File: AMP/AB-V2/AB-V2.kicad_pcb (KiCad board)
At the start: 2 copper layers, 129.9 x 70.2 mm, 52 parts, among them J1 AUX, J3 AUX, P1 WJ500V-5.08-3P, Q1 2SC5200N-OSEN, Q13 BD140, Q14 BD140, Q15 BD139, Q16 BD139, Q17 BD140, Q18 BD140, Q2 2SC5200N-OSEN, Q21 BD139, U1 CYA0630-4.7UH

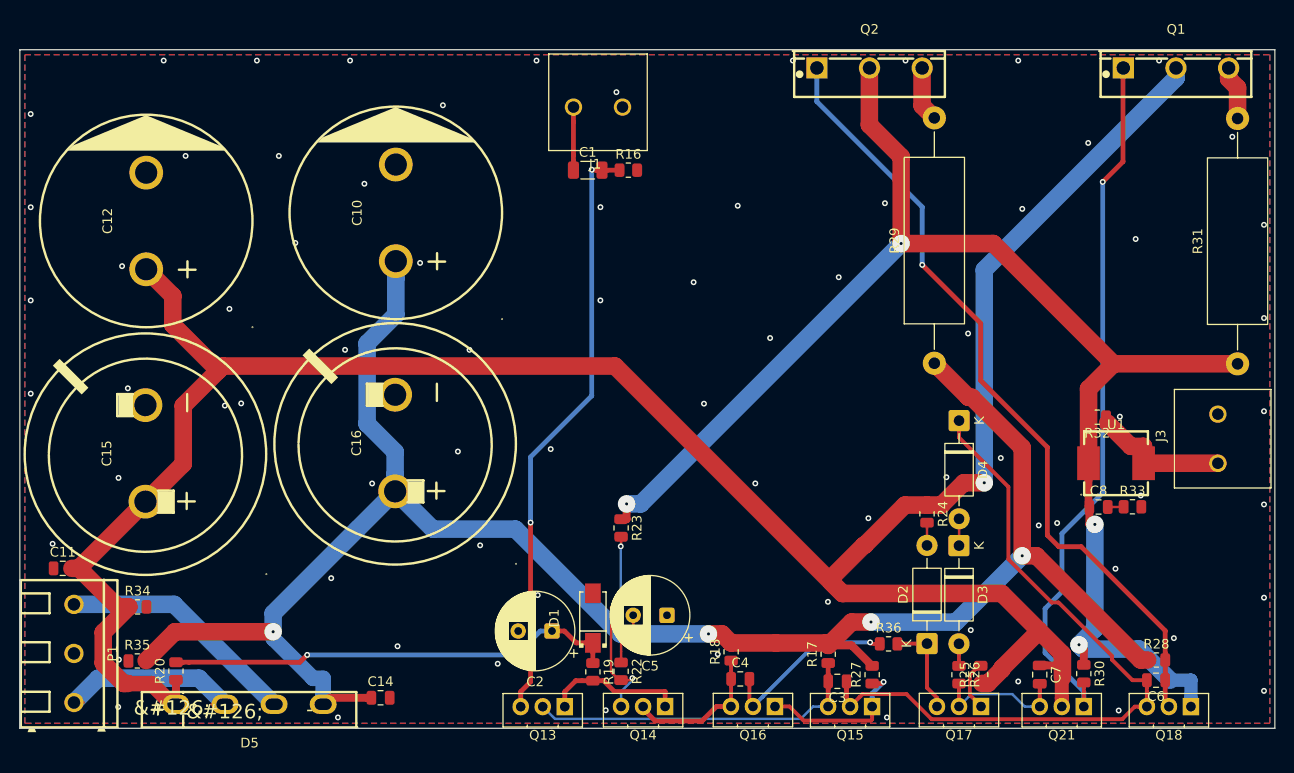
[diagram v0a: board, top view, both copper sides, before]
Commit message: kfahh
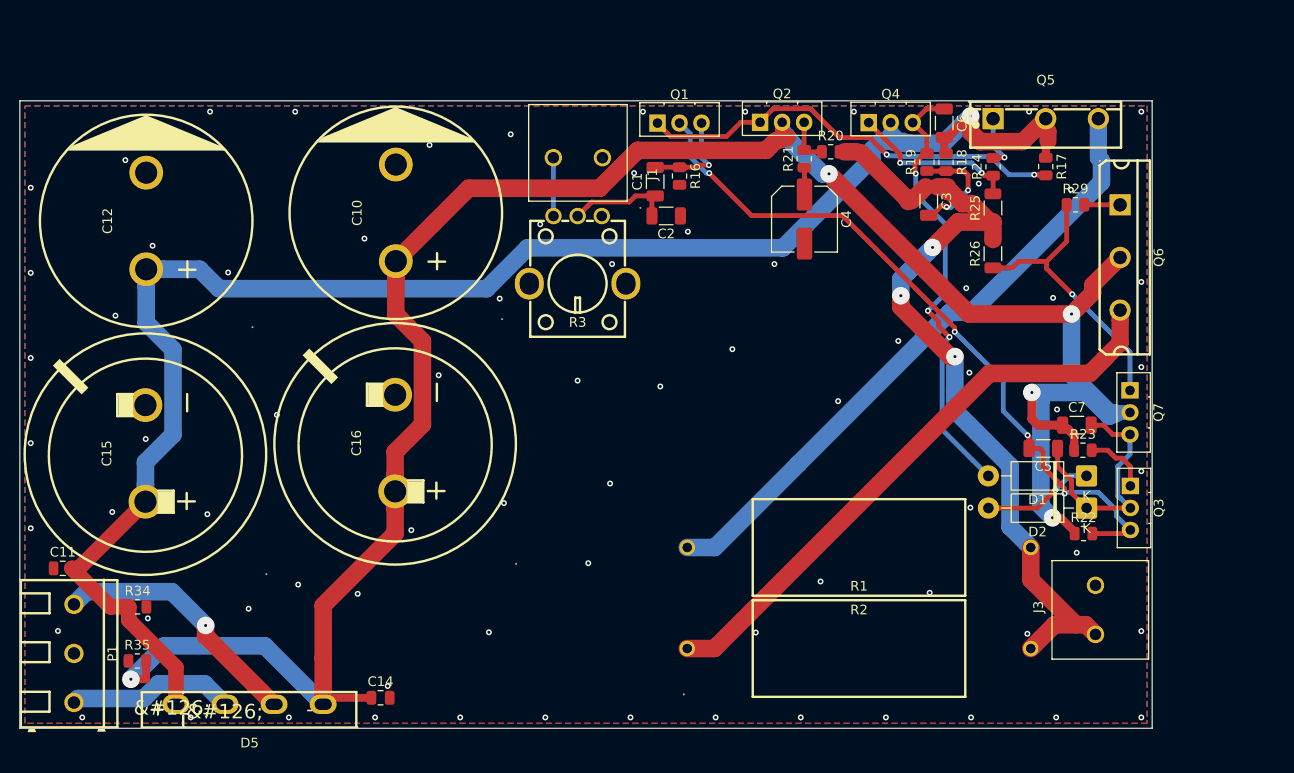
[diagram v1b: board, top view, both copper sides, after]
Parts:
- removed C8: 100 nF, Capacitor_SMD:C_0805_2012Metric
- removed D3, D4: 1N4007, Diode_THT:D_DO-41_SOD81_P10.16mm_Horizontal
- removed Q13, Q14, Q17, Q18: BD140, Package_TO_SOT_THT:TO-126-3_Vertical
- removed Q15, Q16, Q21: BD139, Package_TO_SOT_THT:TO-126-3_Vertical
- removed R27: 150, Resistor_SMD:R_0805_2012Metric
- removed R28, R30: 100, Resistor_SMD:R_0805_2012Metric
- removed R31: 0.47, Resistor_THT:R_Axial_DIN0617_L17.0mm_D6.0mm_P25.40mm_Horizontal
- removed R32, R33: 10, Resistor_SMD:R_0805_2012Metric
- removed R36: 10k, Resistor_SMD:R_0805_2012Metric
- removed U1: CYA0630-4.7UH, lcsc_footprints:C5189748_IND-SMD_L7_2-W6_6_GPSR07X0
- added Q3: BD139, Package_TO_SOT_THT:TO-126-3_Vertical, F.Cu at (245.0, 85.0)
- added Q4: BD139, Package_TO_SOT_THT:TO-126-3_Vertical, F.Cu at (217.9, 47.4)
- added Q5: 2SC5200N-OSEN, lcsc_footprints:C49055716_TO-3P-3_L15_6-W4_8-P5_45-L, F.Cu at (236.2, 47.0)
- added Q6: 2SA1943-O(Q, lcsc_footprints:C545244_TO-3PL_L20_0-W5_0-P5_45-L_1, F.Cu at (243.9, 61.4)
- added Q7: BD140, Package_TO_SOT_THT:TO-126-3_Vertical, F.Cu at (244.9, 75.2)
- added R1: CR-L5W-0.33ΩJ, lcsc_footprints:C334290_RES-TH_BD9_5-L22_0-P26_00-D0_7, F.Cu at (216.9, 91.4)
- added R2: CR-L5W-0.33ΩJ, lcsc_footprints:C334290_RES-TH_BD9_5-L22_0-P26_00-D0_7, F.Cu at (216.9, 101.9)
- added R21: 470, Resistor_SMD:R_0805_2012Metric, F.Cu at (211.2, 51.2)
- added R3: RK09K1130A70, lcsc_footprints:C351173_RES-TH_RK09K1130A70, F.Cu at (187.8, 60.6)
- C1: value 2.2 uF -> 10 uF
- C2, C5: value 100 uF -> 100 pF; footprint Capacitor_THT:CP_Radial_D8.0mm_P3.50mm -> Capacitor_SMD:C_1206_3216Metric
- C3: value 10 pF -> 10 uF; footprint Capacitor_SMD:C_0805_2012Metric -> Capacitor_SMD:C_1206_3216Metric
- C4: value 10 pF -> 100 uF; footprint Capacitor_SMD:C_0805_2012Metric -> Capacitor_SMD:C_Elec_6.3x7.7
- C6, C7: value 1 nF -> 470 pF; footprint Capacitor_SMD:C_0805_2012Metric -> Capacitor_SMD:C_1206_3216Metric
- D1: value 1SMA4749A -> 1N4007; footprint lcsc_footprints:C173489_SMA_L4_4-W2_8-LS5_4-RD -> Diode_THT:D_DO-41_SOD81_P10.16mm_Horizontal
- Q1, Q2: value 2SC5200N-OSEN -> BD140; footprint lcsc_footprints:C49055716_TO-3P-3_L15_6-W4_8-P5_45-L -> Package_TO_SOT_THT:TO-126-3_Vertical
- R17: value 3.3k -> 22k
- R19: value 33k -> 3.3k
- R20: value 4.7k -> 22k
- R22: value 1k -> 1.5k
- R23: value 68k -> 33
- R24: value 150 -> 10
- R25: value 150 -> 100; footprint Resistor_SMD:R_0805_2012Metric -> Resistor_SMD:R_1206_3216Metric
- R26: value 33 -> 100; footprint Resistor_SMD:R_0805_2012Metric -> Resistor_SMD:R_1206_3216Metric
- R29: value 0.47 -> 10; footprint Resistor_THT:R_Axial_DIN0617_L17.0mm_D6.0mm_P25.40mm_Horizontal -> Resistor_SMD:R_0805_2012Metric
- moved R20 86.5 mm to (214.0, 50.5), turned to 0 degrees
- moved R19 63.1 mm to (223.9, 51.5), turned to 90 degrees
- moved C6 61.7 mm to (225.7, 47.5), turned to -90 degrees
- moved R18 55.3 mm to (225.9, 51.5), turned to -90 degrees
- moved R17 55.3 mm to (236.2, 52.0), turned to -90 degrees
- moved Q1 54.0 mm to (196.0, 47.5)
- moved D1 53.2 mm to (240.4, 84.0), turned to 180 degrees
- moved C3 50.6 mm to (224.1, 55.6), turned to -90 degrees
- moved R22 50.0 mm to (240.1, 90.0), turned to 0 degrees
- moved R23 48.5 mm to (240.1, 81.3), turned to 0 degrees
- moved R25 48.3 mm to (230.8, 56.3)
- moved C4 48.1 mm to (211.2, 57.4), turned to -90 degrees
- moved C2 44.6 mm to (196.9, 57.1)
- moved R26 43.7 mm to (230.8, 61.0), turned to 90 degrees
- moved C5 42.6 mm to (236.0, 81.2)
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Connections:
- C1 pad 2: Net-(Q13-B) -> Net-(Q1-B)
- C2 pad 1: Net-(D1-K) -> GND
- C2 pad 2: GND -> /IN
- C3 pad 1: Net-(D4-K) -> /OUT
- C3 pad 2: Net-(Q13-C) -> Net-(C3-Pad2)
- C4 pad 1: Net-(Q14-C) -> Net-(C4-Pad1)
- C4 pad 2: Net-(Q16-C) -> GND
- C5 pad 1: GND -> Net-(D2-K)
- C5 pad 2: Net-(C5-Pad2) -> Net-(Q1-C)
- C6 pad 1: Net-(Q18-C) -> Net-(D1-A)
- C6 pad 2: Net-(D4-K) -> +VDC
- C7 pad 1: +VDC -> -VDC
- C7 pad 2: Net-(Q17-C) -> Net-(D2-K)
- D1 pad 2: GND -> Net-(D1-A)
- D2 pad 2: Net-(D2-A) -> Net-(D1-K)
- J1 pad 2: /IN -> Net-(J1-Pin_2)
- Q1 pad 1: Net-(Q1-B) -> Net-(Q1-E)
- Q1 pad 2: +VDC -> Net-(Q1-C)
- Q1 pad 3: Net-(Q1-E) -> Net-(Q1-B)
- Q2 pad 1: Net-(Q18-C) -> Net-(Q1-E)
- Q2 pad 2: Net-(Q18-E) -> -VDC
- Q2 pad 3: Net-(Q2-E) -> Net-(Q2-B)
- R16 pad 1: Net-(Q13-B) -> Net-(Q1-B)
- R17 pad 1: Net-(Q13-C) -> +VDC
- R17 pad 2: -VDC -> Net-(Q1-E)
- R18 pad 1: Net-(Q14-C) -> +VDC
- R18 pad 2: -VDC -> Net-(C3-Pad2)
- R19 pad 1: Net-(D1-K) -> Net-(C3-Pad2)
- R19 pad 2: Net-(Q13-E) -> Net-(D1-A)
- R20 pad 1: +VDC -> Net-(Q2-B)
- R20 pad 2: Net-(D1-K) -> /OUT
- R22 pad 1: Net-(C5-Pad2) -> -VDC
- R22 pad 2: Net-(Q14-B) -> Net-(Q1-C)
- R23 pad 1: Net-(Q18-E) -> -VDC
- R23 pad 2: Net-(Q14-B) -> Net-(Q3-E)
- R24 pad 1: +VDC -> Net-(Q4-E)
- R24 pad 2: Net-(D2-A) -> Net-(Q5-B)
- R25 pad 1: +VDC -> /OUT
- R25 pad 2: Net-(Q17-E) -> Net-(Q4-E)
- R26 pad 1: Net-(D3-A) -> Net-(Q7-E)
- R26 pad 2: Net-(Q17-C) -> /OUT
- R29 pad 1: -VDC -> Net-(Q7-E)
- R29 pad 2: Net-(Q2-E) -> Net-(Q6-B)
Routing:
- net Net-(Q18-E): track 156.0 -> 0.00 mm, vias 4 -> 0
- net Net-(Q18-C): track 82.6 -> 0.00 mm, vias 1 -> 0
- net +VDC: track 257.0 -> 175.8 mm
- net Net-(D4-K): track 74.6 -> 0.00 mm
- net Net-(Q1-C): track 0.00 -> 74.1 mm, vias 0 -> 4
- net /OUT: track 14.4 -> 87.4 mm, vias 0 -> 3
- net Net-(Q5-E): track 0.00 -> 65.3 mm
- net Net-(Q1-B): track 73.6 -> 10.3 mm
- net Net-(Q13-B): track 61.5 -> 0.00 mm, vias 2 -> 0
- net Net-(Q6-E): track 0.00 -> 61.3 mm
- net Net-(D1-A): track 0.00 -> 46.9 mm, vias 0 -> 3
- net Net-(Q1-E): track 5.61 -> 44.8 mm, vias 0 -> 2
- net Net-(D1-K): track 47.1 -> 11.5 mm
- net Net-(Q13-C): track 35.1 -> 0.00 mm
- net -VDC: track 198.3 -> 228.2 mm, vias 4 -> 5
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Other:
- board size 129.9 x 70.2 mm -> 117.2 x 65 mm
